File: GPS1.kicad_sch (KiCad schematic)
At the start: 12 parts, among them J7 GPS_ANT_0, U4 MAX-M10S-00B

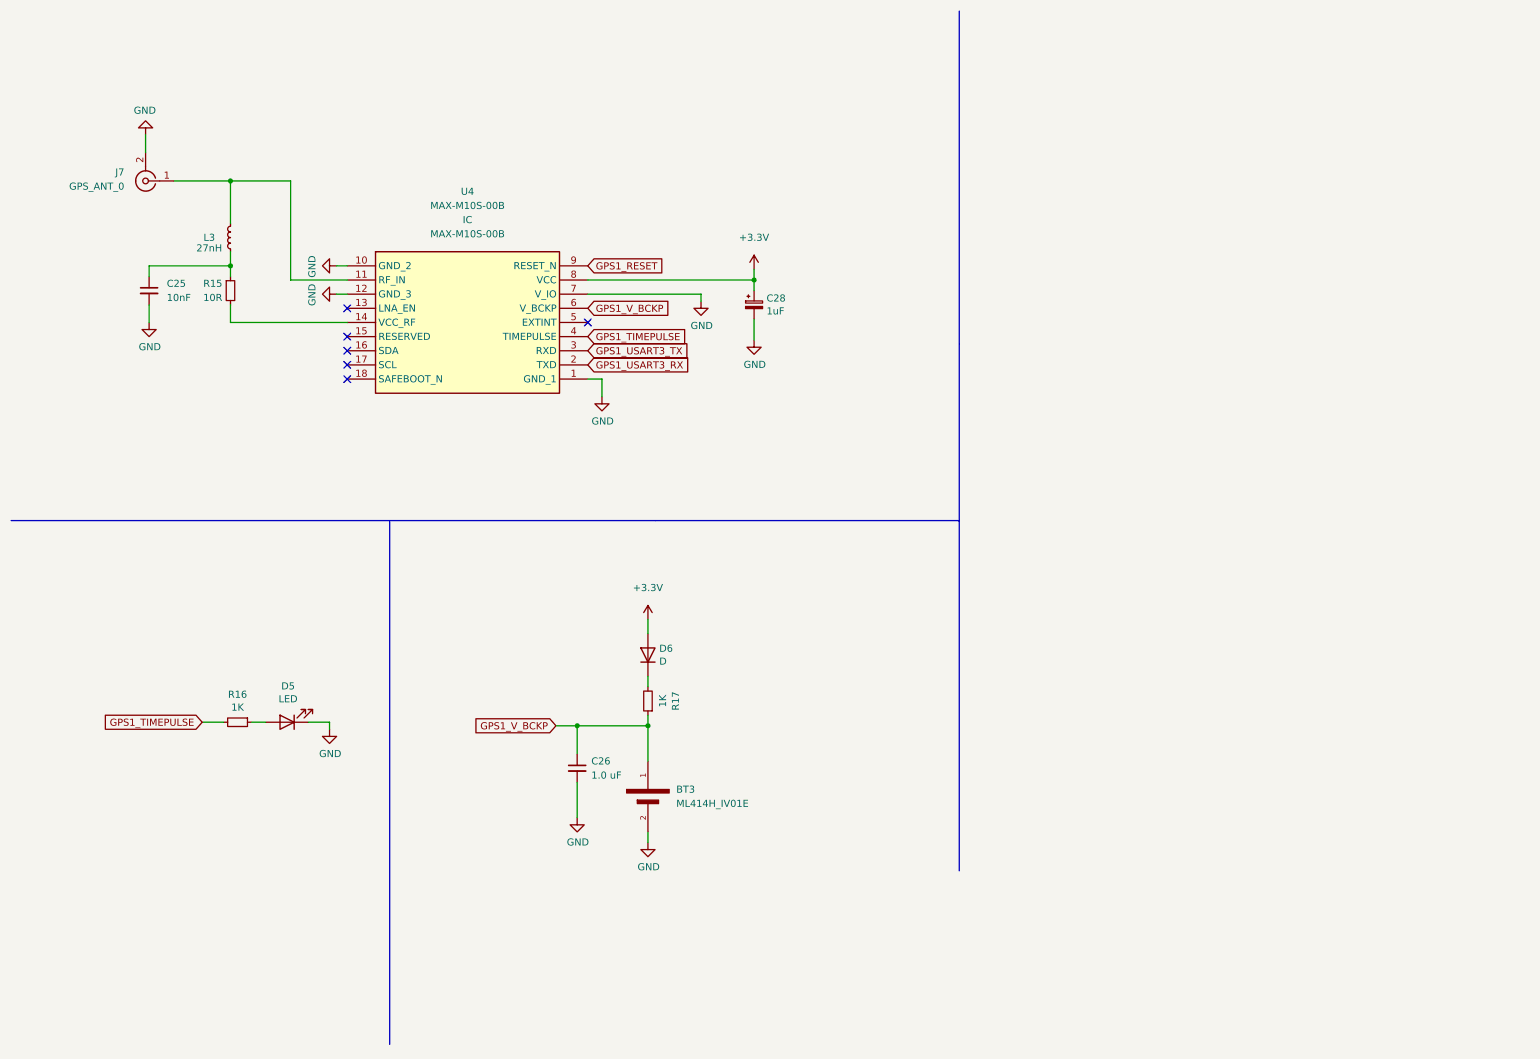
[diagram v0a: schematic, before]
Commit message: Last commit
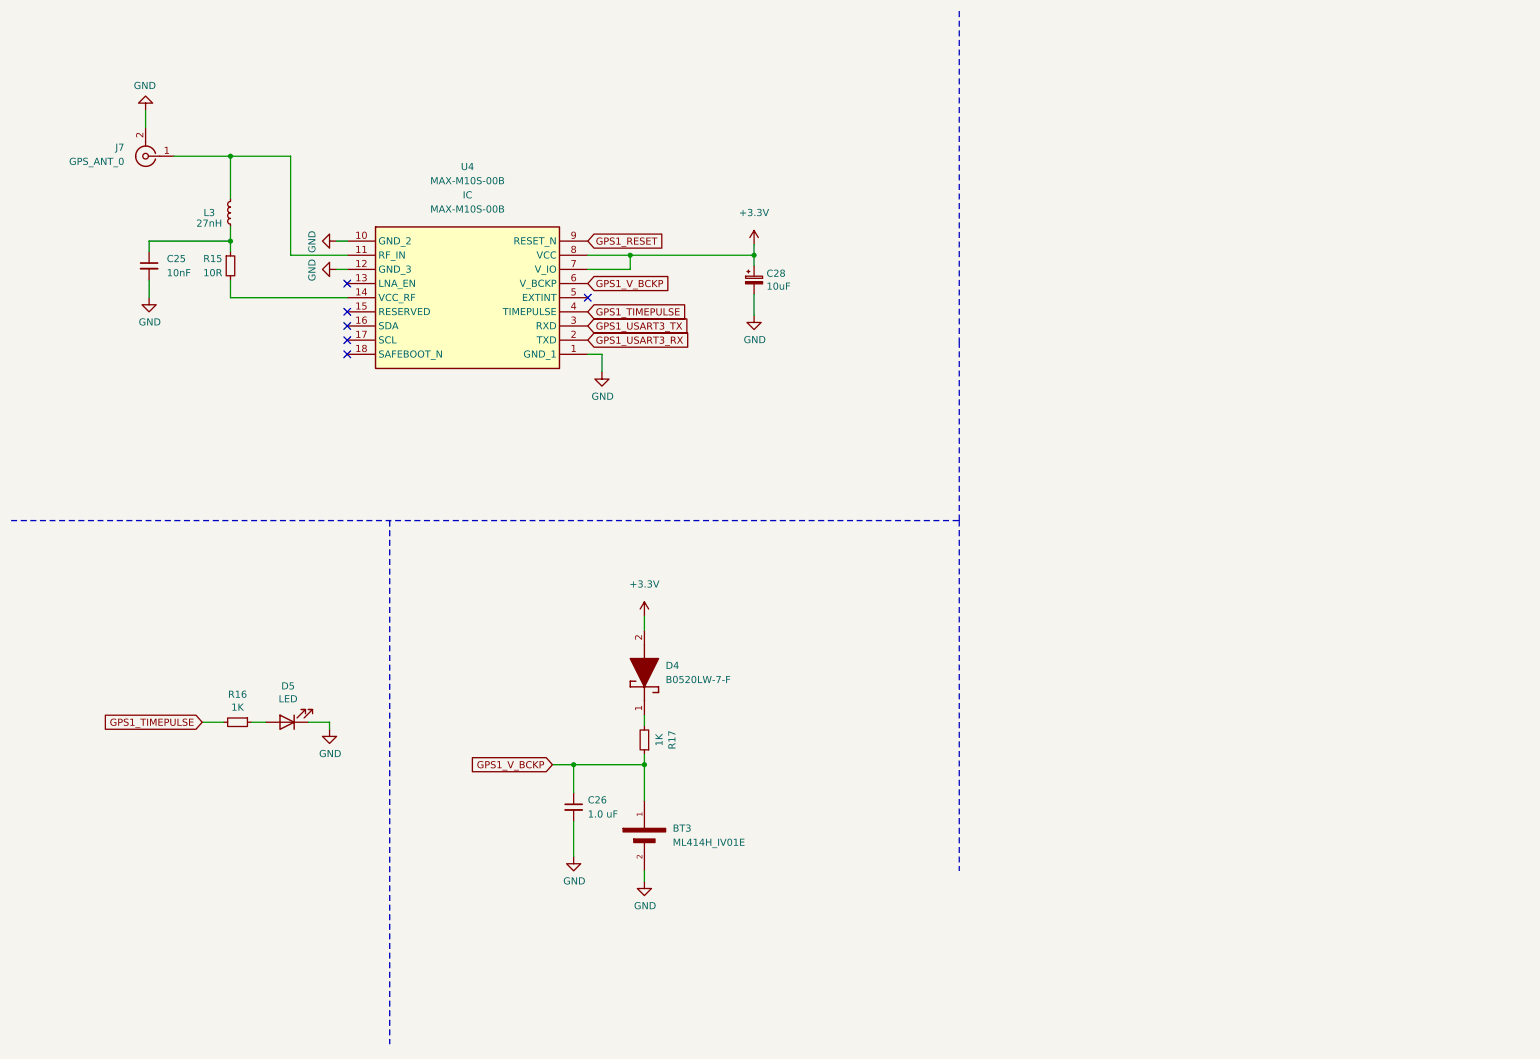
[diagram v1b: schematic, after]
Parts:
- removed D6: D, Diode_SMD:D_1206_3216Metric_Pad1.42x1.75mm_HandSolder, symbol Device:D
- added D4: B0520LW-7-F, B0520LW-7-F:SOD3716X145N, symbol B0520LW-7-F:B0520LW-7-F
- C28: value 1uF -> 10uF; footprint Capacitor_Tantalum_SMD:CP_EIA-3528-21_Kemet-B_Pad1.50x2.35mm_HandSolder -> Capacitor_SMD:C_1210_3225Metric
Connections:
- net +3.3V: now also U4.7 (V_IO), D4.2 (A)
- net GND: no longer U4.7 (V_IO)
- net at R17.2: now also D4.1 (K)
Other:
- moved on the sheet: BT3, C25, C26, C28, J7, L3, R15, R17, U4

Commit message: Second commit
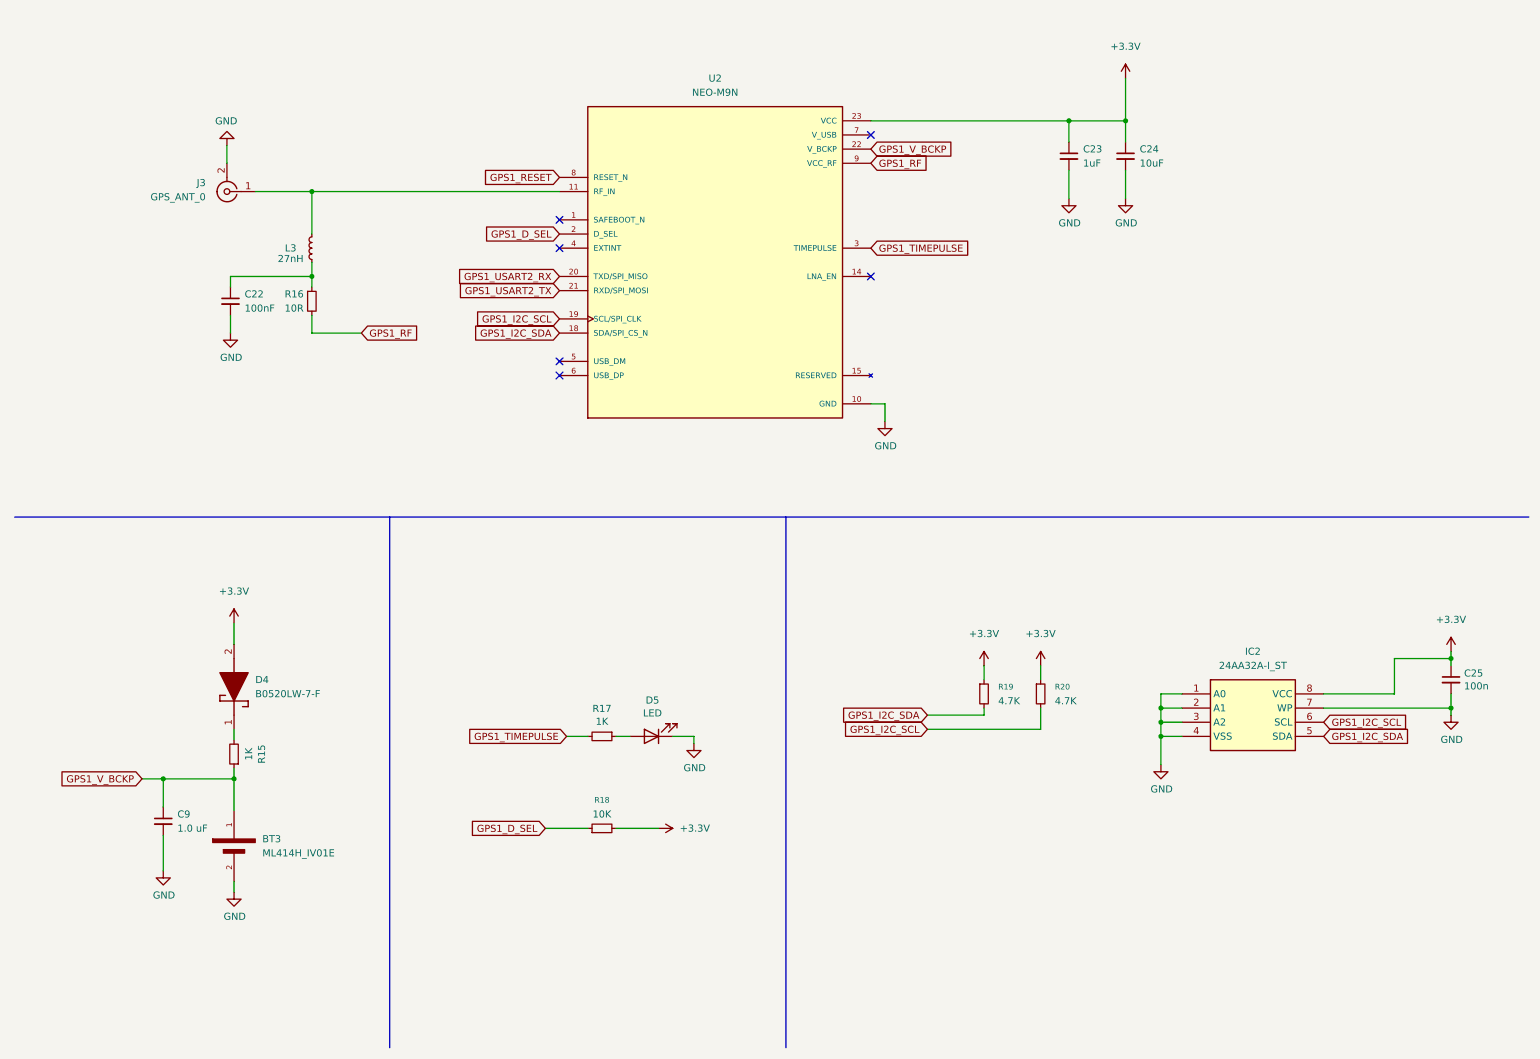
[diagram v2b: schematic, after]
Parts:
- removed C26: 1.0 uF, Capacitor_SMD:C_0805_2012Metric, symbol Device:C_Small
- removed C28: 10uF, Capacitor_SMD:C_1210_3225Metric, symbol Device:CP_Small
- removed J7: GPS_ANT_0, Connector_Coaxial:SMA_Samtec_SMA-J-P-X-ST-EM1_EdgeMount, symbol Connector:Conn_Coaxial
- removed U4: MAX-M10S-00B, MAX-M10S-00B:MAXM10S00B, symbol MAX-M10S-00B:MAX-M10S-00B
- added C22: 100nF, Capacitor_SMD:C_0402_1005Metric, symbol Device:C_Small
- added C23: 1uF, Capacitor_SMD:C_1210_3225Metric, symbol Device:C_Small
- added C24: 10uF, Capacitor_SMD:C_1210_3225Metric, symbol Device:C_Small
- added C9: 1.0 uF, Capacitor_SMD:C_0805_2012Metric, symbol Device:C_Small
- added IC2: 24AA32A-I_ST, 24AA32A-I_ST:SOP65P640X120-8N, symbol 24AA32A-I_ST:24AA32A-I_ST
- added J3: GPS_ANT_0, Connector_Coaxial:SMA_Samtec_SMA-J-P-H-ST-EM1_EdgeMount, symbol Connector:Conn_Coaxial
- added R18: 10K, Resistor_SMD:R_0402_1005Metric, symbol Device:R_Small
- added R19, R20: 4.7K, Resistor_SMD:R_0402_1005Metric, symbol Device:R_Small
- added U2: NEO-M9N, NEO-M9N:XCVR_NEO-M9N, symbol NEO-M9N:NEO-M9N
- BT3: footprint ML414H_IV01E:SEIKO_ML414H_IV01E -> ML414H IV01E:SEIKO_ML414H_IV01E
- C25: value 10nF -> 100n
- R15: value 10R -> 1K; footprint Resistor_SMD:R_0402_1005Metric -> Resistor_SMD:R_0805_2012Metric
- R16: value 1K -> 10R; footprint Resistor_SMD:R_0805_2012Metric -> Resistor_SMD:R_0402_1005Metric
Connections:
- net +3.3V: now also C25.1, C23.1, C24.1, IC2.8 (VCC), R18.2, R19.1, R20.1, U2.23 (VCC)
- net GND: now also C22.2, C23.2, C24.2, C9.2, IC2.1 (A0), IC2.2 (A1), IC2.3 (A2), IC2.4 (VSS), IC2.7 (WP), J3.2 (Ext), U2.10 (GND), U2.12 (GND), U2.13 (GND), U2.24 (GND)
- net GPS1_RESET: now also U2.8 (RESET_N)
- net GPS1_TIMEPULSE: now also R17.2, U2.3 (TIMEPULSE); no longer R16.2
- net GPS1_V_BCKP: now also R15.1, C9.1, U2.22 (V_BCKP); no longer R17.1
- net at R16.1: now also L3.1, C22.1; no longer D5.2 (A)
- net at R15.2: now also D4.1 (K)
- net at L3.2: now also J3.1 (In), U2.11 (RF_IN)
- new net: D5.2 (A), R17.1
- new net: U2.15 (RESERVED), U2.16 (RESERVED), U2.17 (RESERVED)
- new net GPS1_D_SEL: R18.1, U2.2 (D_SEL)
- new net GPS1_I2C_SCL: IC2.6 (SCL), R20.2, U2.19 (SCL/SPI_CLK)
- new net GPS1_I2C_SDA: IC2.5 (SDA), R19.2, U2.18 (SDA/SPI_CS_N)
- new net GPS1_RF: R16.2, U2.9 (VCC_RF)
- new net GPS1_USART2_RX: U2.20 (TXD/SPI_MISO)
- new net GPS1_USART2_TX: U2.21 (RXD/SPI_MOSI)
